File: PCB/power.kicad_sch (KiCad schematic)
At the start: 46 parts, among them J1 S2B-PH, J5 USB4105-GF-A, Q1 2N7002, SW2 PWR, U11 TPS3424A11C13ADRLR, U3 BQ24074RGT, U4 TPS63001, U9 USBLC6-2SC6

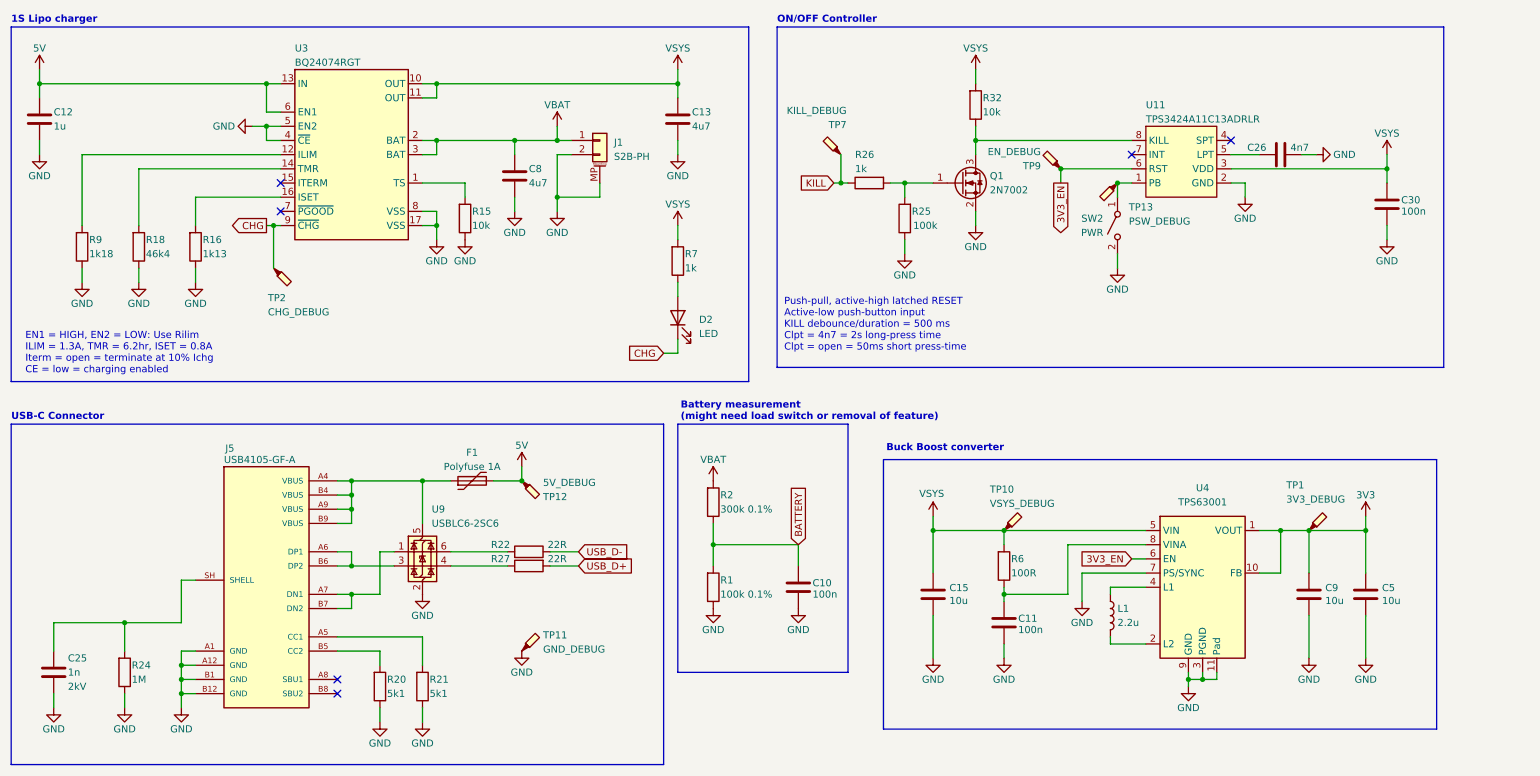
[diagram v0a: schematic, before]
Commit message: Ready for production
Small readability and producability optimizations
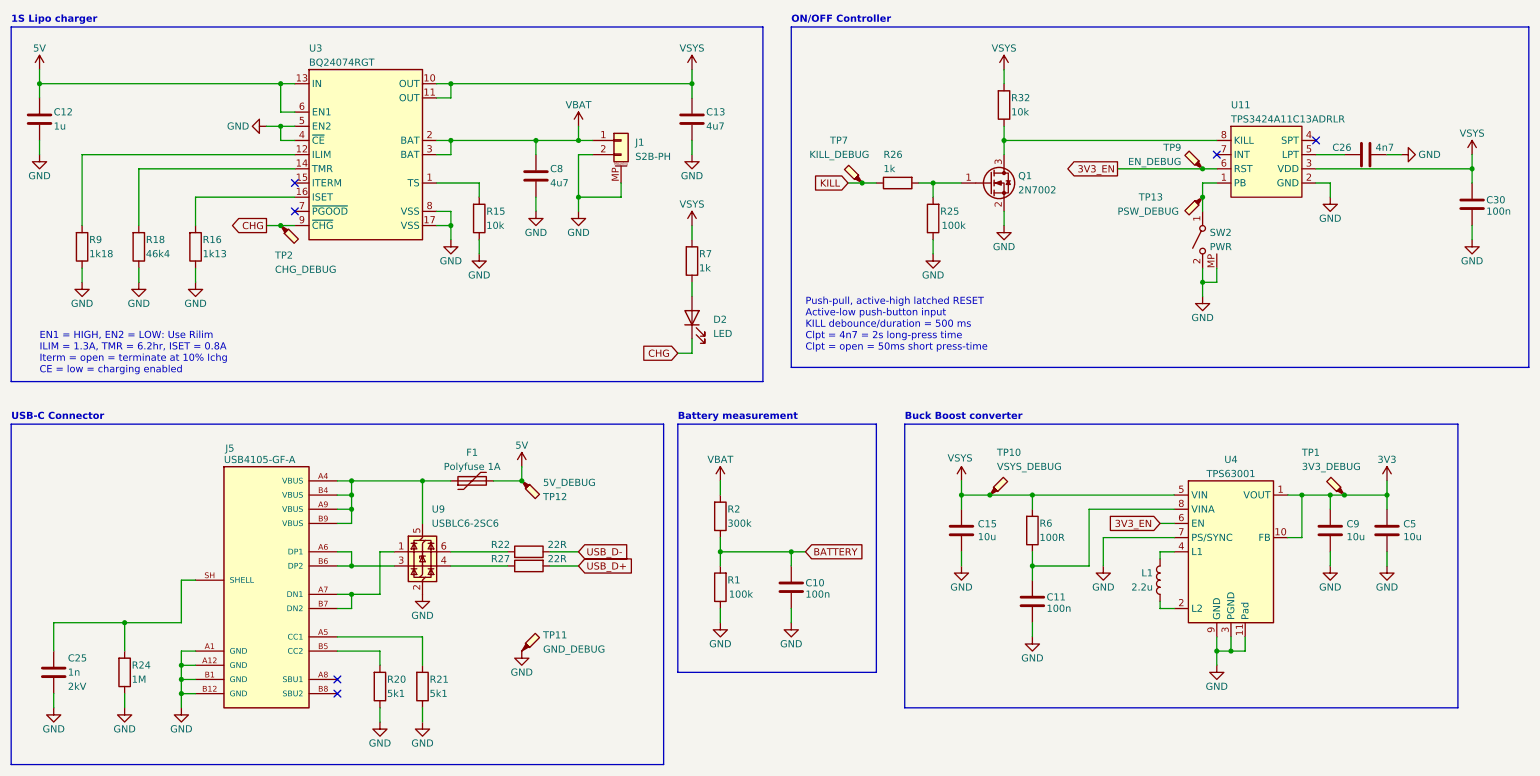
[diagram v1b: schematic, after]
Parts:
- C25: Manufacturer KEMET -> KEMET
- D2: Manifacturer Würth Elektronik -> (none); Manufacturer (none) -> Wurth
- J1: Manufacturer JST Sales America Inc. -> JST
- R1: value 100k 0.1% -> 100k; Digikey YAG1235CT-ND -> 311-100KHRCT-ND; Partnumber RT0603BRD07100KL -> RC0603FR-07100KL
- R2: value 300k 0.1% -> 300k; Digikey YAG1627CT-ND -> 311-300KHRTR-ND; Partnumber RT0603BRD07300KL -> RC0603FR-07300KL
- R20, R21: Digikey YAG3621CT-ND -> 311-5.10KHRTR-ND; Partnumber AC0603FR-075K1L -> RC0603FR-075K1L
- R22, R27: Digikey YAG3581CT-ND -> 311-22.0HRTR-ND; Partnumber AC0603FR-0722RL -> RC0603FR-0722RL
- U9: Digikey 5399-USBLC6-2SC6CT-ND -> 497-5235-2-ND; Manufacturer Shenzhen Slkormicro Semicon Co., Ltd. -> STMicroelectronics
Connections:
- net GND: now also SW2.MP
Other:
- note added: "Battery measurement"
- note removed: "Battery measurement (might need load switch or removal of feature)"
- moved on the sheet: C10, C11, C13, C15, C26, C30, C5, C8, C9, D2, J1, L1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
